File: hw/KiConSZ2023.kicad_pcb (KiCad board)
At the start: 4 copper layers, 100 x 60 mm, 108 parts, among them J2 Conn_01x06, J3 USB_C_Receptacle_USB2.0, J4 Conn_02x03_Top_Bottom, J5 Conn_02x03_Top_Bottom, J6 BM20B(0.8)-10DS-0.4V, Q10 SK2302AAT, Q11 SK2302AAT, Q12 SK2302AAT, Q13 SK2302AAT, Q14 SK2302AAT, Q15 SK2302AAT, Q16 SK2302AAT, Q17 SK2302AAT, Q2 SK2302AAT, Q3 SK2302AAT, Q4 SK2302AAT, Q5 SK2302AAT, Q6 SK2302AAT, Q7 SK2302AAT, Q8 SK2302AAT, Q9 SK2302AAT, SW2 SKRPACE010, SW3 SKRPACE010, SW4 SW_SPDT, U2 N32L406RBL7, U3 PUSB3FR4, U4 SY8088IAAC, U5 ME2118C33M5G

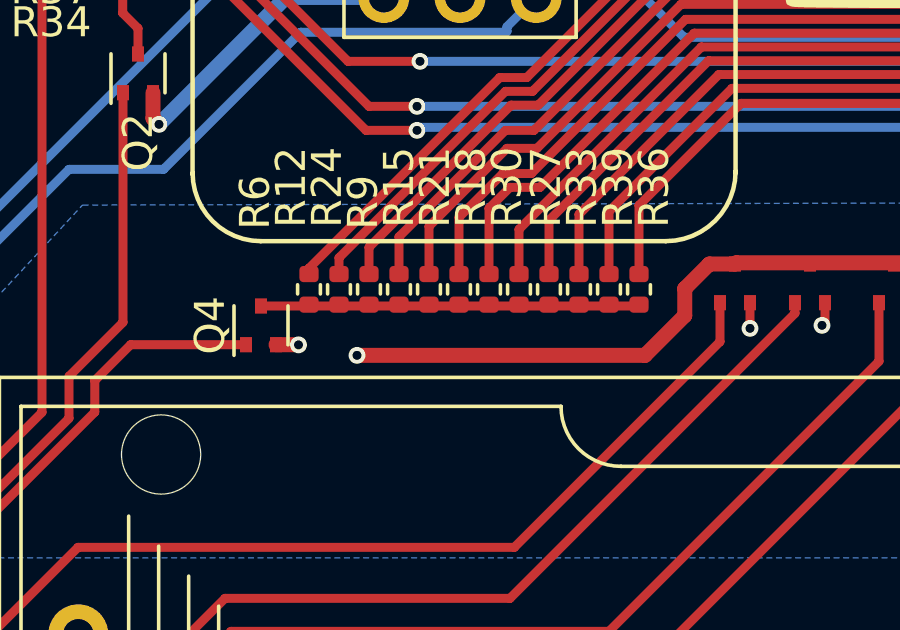
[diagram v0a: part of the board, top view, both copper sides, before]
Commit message: updated track
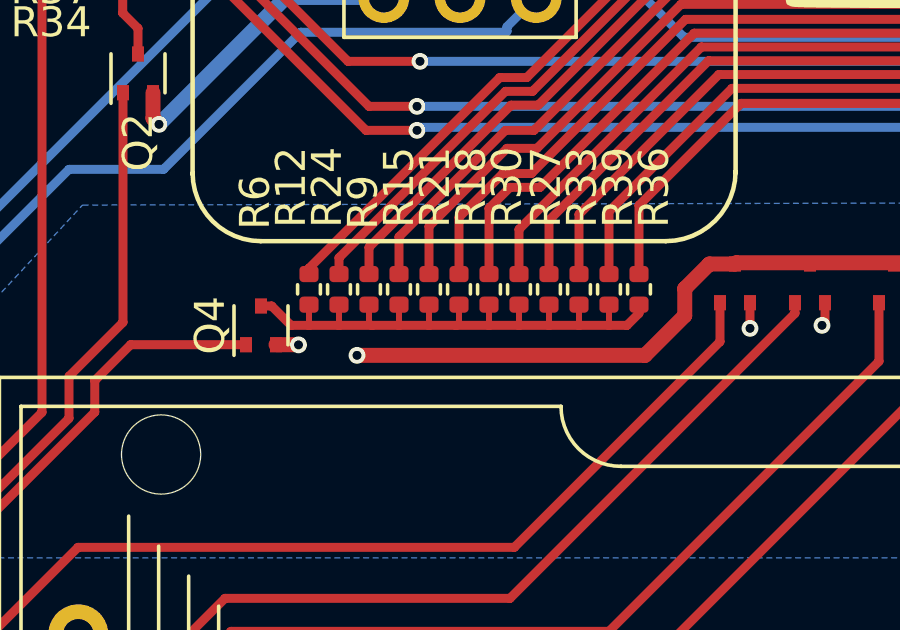
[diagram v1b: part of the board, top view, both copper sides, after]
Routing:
- net /LED Row/LowSide_Input_Source_B: track 12.6 -> 21.0 mm
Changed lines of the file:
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@@
   (segment (start 93.265 95.59) (end 95.15 95.59) (width 0.3) (layer "F.Cu") (net 46))
   (segment (start 93.25 95.605) (end 93.265 95.59) (width 0.3) (layer "F.Cu") (net 46))
-  (segment (start 88.4 119.955) (end 100.955 119.955) (width 0.3) (layer "F.Cu") (net 47))
-  (segment (start 100.955 119.955) (end 101 119.91) (width 0.3) (layer "F.Cu") (net 47))
+  (segment (start 90 120.6) (end 91 120.6) (width 0.3) (layer "F.Cu") (net 47))
+  (segment (start 88.755 119.955) (end 89.4 120.6) (width 0.3) (layer "F.Cu") (net 47))
+  (segment (start 100 119.91) (end 100 120.6) (width 0.2) (layer "F.Cu") (net 47))
+  (segment (start 99 119.91) (end 99 120.6) (width 0.2) (layer "F.Cu") (net 47))
+  (segment (start 98 119.91) (end 98 120.6) (width 0.2) (layer "F.Cu") (net 47))
+  (segment (start 90 119.91) (end 90 120.6) (width 0.2) (layer "F.Cu") (net 47))
+  (segment (start 91 120.6) (end 92.1 120.6) (width 0.3) (layer "F.Cu") (net 47))
+  (segment (start 100.6 120.6) (end 101 120.2) (width 0.3) (layer "F.Cu") (net 47))
+  (segment (start 96 119.91) (end 96 120.6) (width 0.2) (layer "F.Cu") (net 47))
+  (segment (start 101 120.2) (end 101 119.91) (width 0.3) (layer "F.Cu") (net 47))
+  (segment (start 97 120.6) (end 98 120.6) (width 0.3) (layer "F.Cu") (net 47))
+  (segment (start 88.4 119.955) (end 88.755 119.955) (width 0.3) (layer "F.Cu") (net 47))
+  (segment (start 89.4 120.6) (end 90 120.6) (width 0.3) (layer "F.Cu") (net 47))
+  (segment (start 92.1 120.6) (end 93 120.6) (width 0.3) (layer "F.Cu") (net 47))
+  (segment (start 99 120.6) (end 100 120.6) (width 0.3) (layer "F.Cu") (net 47))
+  (segment (start 97 119.91) (end 97 120.6) (width 0.2) (layer "F.Cu") (net 47))
+  (segment (start 96 120.6) (end 97 120.6) (width 0.3) (layer "F.Cu") (net 47))
+  (segment (start 100 120.6) (end 100.6 120.6) (width 0.3) (layer "F.Cu") (net 47))
+  (segment (start 93 119.91) (end 93 120.6) (width 0.2) (layer "F.Cu") (net 47))
+  (segment (start 98 120.6) (end 99 120.6) (width 0.3) (layer "F.Cu") (net 47))
+  (segment (start 91 119.91) (end 91 120.6) (width 0.2) (layer "F.Cu") (net 47))
+  (segment (start 94 120.6) (end 94.9 120.6) (width 0.3) (layer "F.Cu") (net 47))
+  (segment (start 92 119.91) (end 92 120.5) (width 0.2) (layer "F.Cu") (net 47))
+  (segment (start 95 120.5) (end 94.9 120.6) (width 0.2) (layer "F.Cu") (net 47))
+  (segment (start 94.9 120.6) (end 96 120.6) (width 0.3) (layer "F.Cu") (net 47))
+  (segment (start 94 119.91) (end 94 120.6) (width 0.2) (layer "F.Cu") (net 47))
+  (segment (start 93 120.6) (end 94 120.6) (width 0.3) (layer "F.Cu") (net 47))
+  (segment (start 95 119.91) (end 95 120.5) (width 0.2) (layer "F.Cu") (net 47))
+  (segment (start 92 120.5) (end 92.1 120.6) (width 0.2) (layer "F.Cu") (net 47))
   (segment (start 67.925 115.575) (end 68.975 115.575) (width 0.15) (layer "F.Cu") (net 48))
   (segment (start 67.925 115.575) (end 72.075 115.575) (width 0.15) (layer "F.Cu") (net 48))
